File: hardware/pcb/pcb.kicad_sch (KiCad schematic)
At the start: 4 parts, among them U101 BQ7694003DBTR, U102 HCZZ0520-13, U103 HCZZ0520-13, U104 ESP32-C3

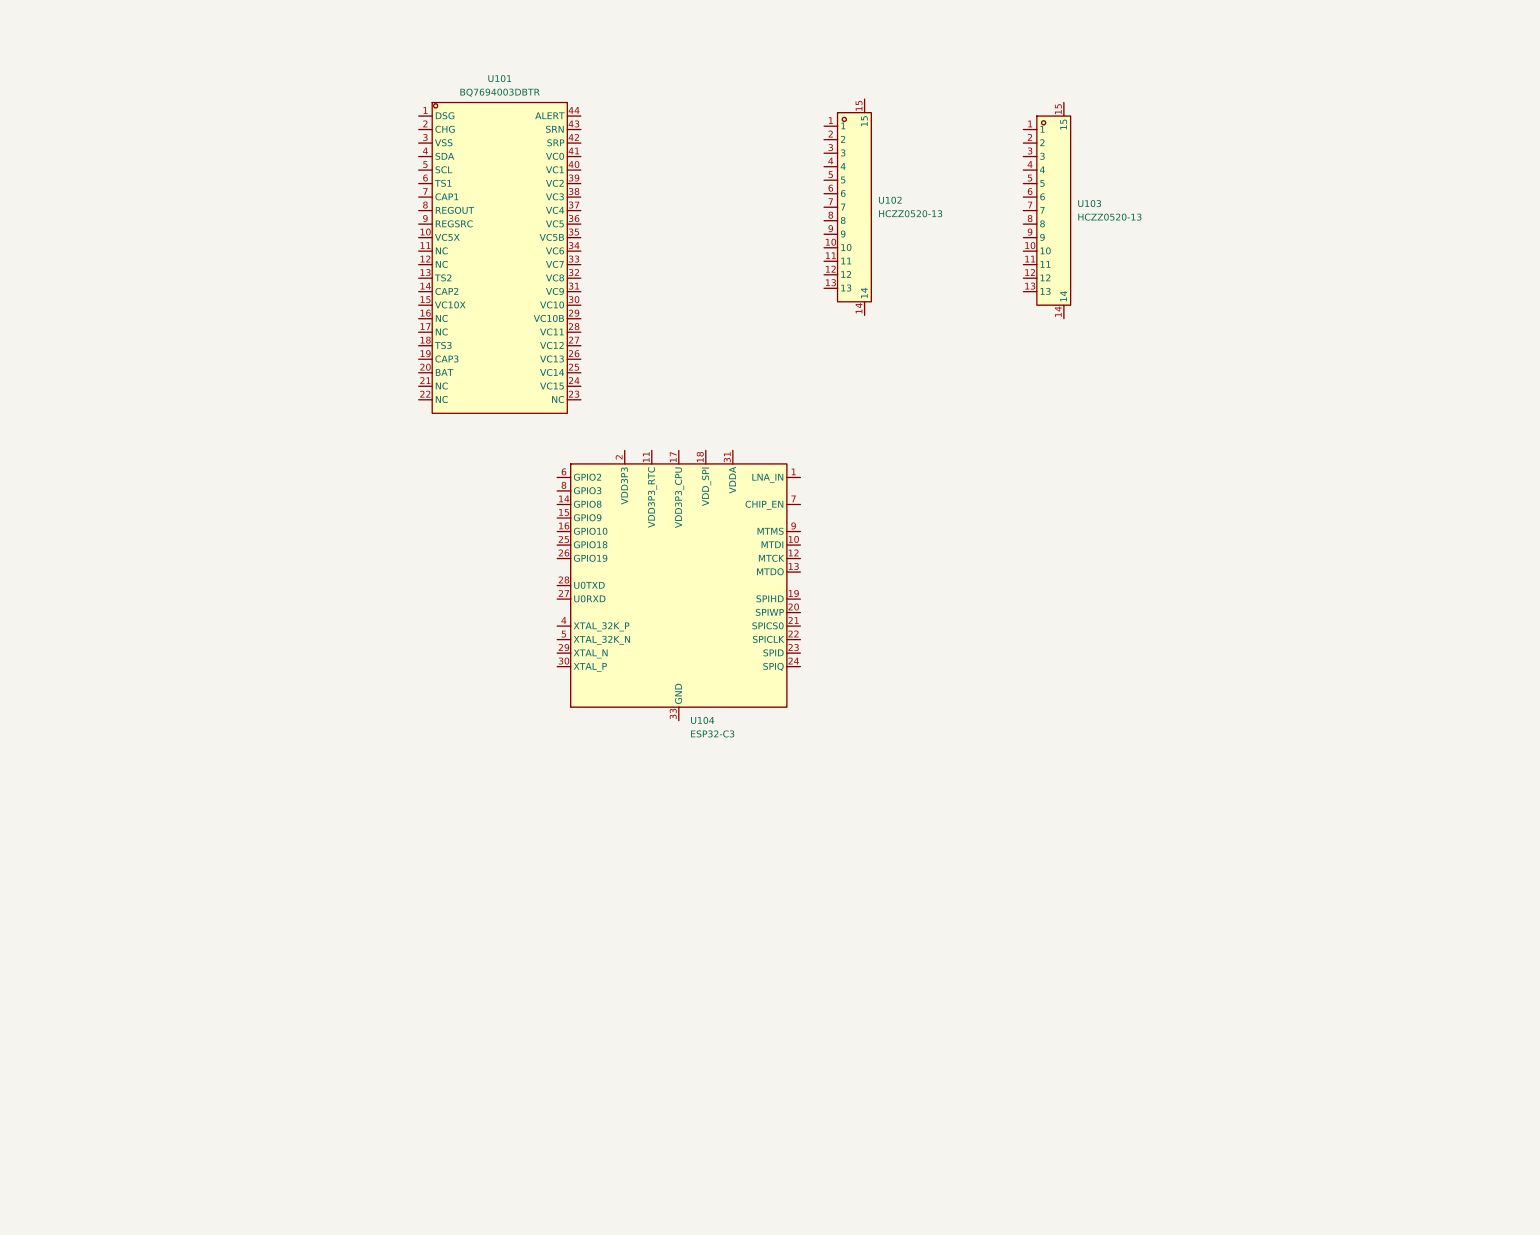
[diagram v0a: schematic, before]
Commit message: re writing the code for better optimization
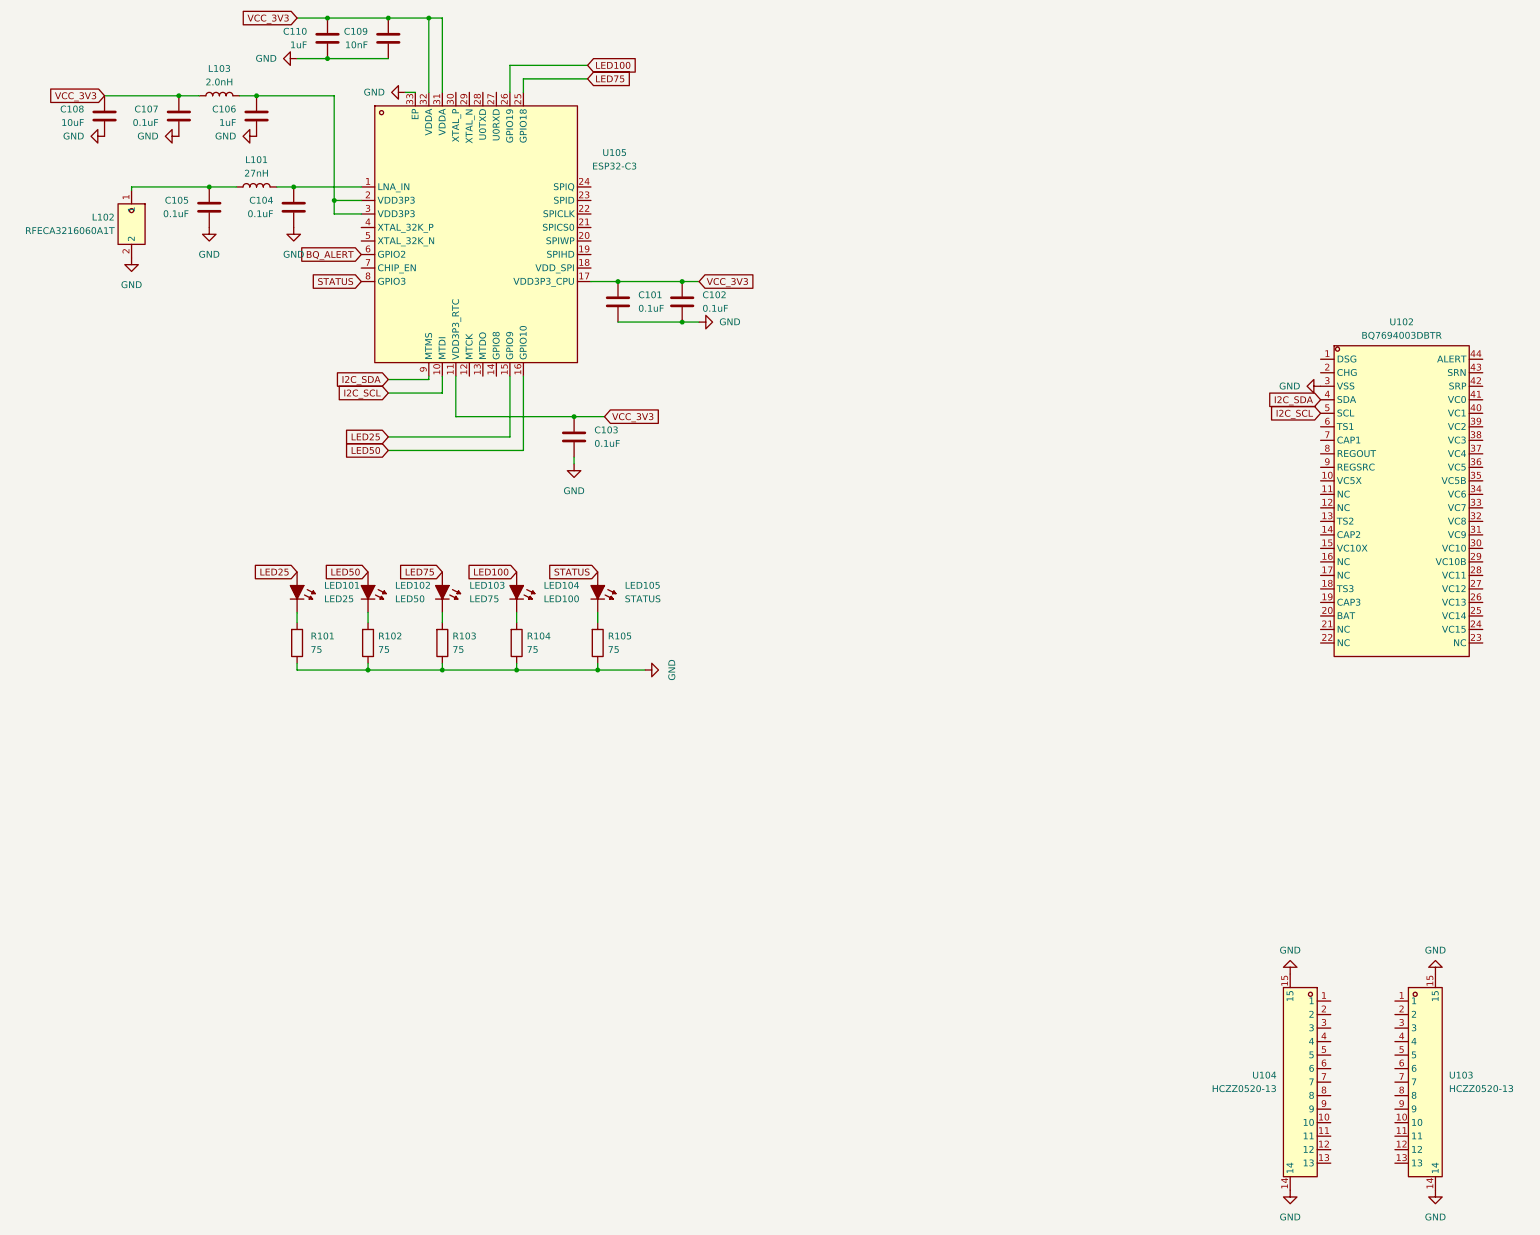
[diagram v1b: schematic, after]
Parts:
- removed U101: BQ7694003DBTR, easyeda2kicad:TSSOP-44_L10.0-W4.4-P0.50-LS6.4-BL-EP, symbol easyeda2kicad:BQ7694003DBTR
- removed U102: HCZZ0520-13, easyeda2kicad:CONN-SMD_13P-P2.50_HCZZ0520-13, symbol easyeda2kicad:HCZZ0520-13
- removed U104: ESP32-C3, Package_DFN_QFN:QFN-32-1EP_5x5mm_P0.5mm_EP3.7x3.7mm, symbol MCU_Espressif:ESP32-C3
- added C101, C102, C103, C104, C105, C107: 0.1uF, PCM_Capacitor_SMD_AKL:C_0402_1005Metric, symbol PCM_Capacitor_AKL:C_0402
- added C106, C110: 1uF, PCM_Capacitor_SMD_AKL:C_0402_1005Metric, symbol PCM_Capacitor_AKL:C_0402
- added C108: 10uF, PCM_Capacitor_SMD_AKL:C_0402_1005Metric, symbol PCM_Capacitor_AKL:C_0402
- added C109: 10nF, PCM_Capacitor_SMD_AKL:C_0402_1005Metric, symbol PCM_Capacitor_AKL:C_0402
- added L101: 27nH, Inductor_SMD:L_1206_3216Metric_Pad1.22x1.90mm_HandSolder, symbol Device:L
- added L102: RFECA3216060A1T, easyeda2kicad:ANT-SMD_L3.1-W1.6, symbol easyeda2kicad:RFECA3216060A1T
- added L103: 2.0nH, Inductor_SMD:L_1206_3216Metric_Pad1.22x1.90mm_HandSolder, symbol Device:L
- added LED101: LED25, PCM_LED_SMD_AKL:LED_0603_1608Metric, symbol PCM_LED_AKL:LED_0603
- added LED102: LED50, PCM_LED_SMD_AKL:LED_0603_1608Metric, symbol PCM_LED_AKL:LED_0603
- added LED103: LED75, PCM_LED_SMD_AKL:LED_0603_1608Metric, symbol PCM_LED_AKL:LED_0603
- added LED104: LED100, PCM_LED_SMD_AKL:LED_0603_1608Metric, symbol PCM_LED_AKL:LED_0603
- added LED105: STATUS, PCM_LED_SMD_AKL:LED_0603_1608Metric, symbol PCM_LED_AKL:LED_0603
- added R101, R102, R103, R104, R105: 75, PCM_Resistor_SMD_AKL:R_0402_1005Metric, symbol PCM_Resistor_AKL:R_0402
- added U102: BQ7694003DBTR, easyeda2kicad:TSSOP-44_L10.0-W4.4-P0.50-LS6.4-BL-EP, symbol easyeda2kicad:BQ7694003DBTR
- added U104: HCZZ0520-13, easyeda2kicad:CONN-SMD_13P-P2.50_HCZZ0520-13, symbol easyeda2kicad:HCZZ0520-13
- added U105: ESP32-C3, easyeda2kicad:QFN-32_L5.0-W5.0-P0.50-TL-EP3.7, symbol easyeda2kicad:ESP32-C3
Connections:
- net GND: now reaches U103.14
- net GND: now also U103.15, C101.2, C102.2, C103.2, C104.2, C105.2, C106.2, C107.2, C108.2, C109.2, C110.2, L102.2, R101.2, R102.2, R103.2, R104.2, R105.2, U102.3 (VSS), U104.14, U104.15, U105.33 (EP)
- new net: LED105.1 (K), R105.1
- new net: LED103.1 (K), R103.1
- new net: C106.1, L103.1, U105.2 (VDD3P3), U105.3 (VDD3P3)
- new net: LED102.1 (K), R102.1
- new net: C104.1, L101.2, U105.1 (LNA_IN)
- new net: C105.1, L101.1, L102.1
- new net: LED101.1 (K), R101.1
- new net: LED104.1 (K), R104.1
- new net BQ_ALERT: U105.6 (GPIO2)
- new net I2C_SCL: U102.5 (SCL), U105.10 (MTDI)
- new net I2C_SDA: U102.4 (SDA), U105.9 (MTMS)
- new net LED100: LED104.2 (A), U105.26 (GPIO19)
- new net LED25: LED101.2 (A), U105.15 (GPIO9)
- new net LED50: LED102.2 (A), U105.16 (GPIO10)
- new net LED75: LED103.2 (A), U105.25 (GPIO18)
- new net STATUS: LED105.2 (A), U105.8 (GPIO3)
- new net VCC_3V3: C101.1, C102.1, C103.1, C107.1, C108.1, C109.1, C110.1, L103.2, U105.11 (VDD3P3_RTC), U105.17 (VDD3P3_CPU), U105.31 (VDDA), U105.32 (VDDA)

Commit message: readme done and eveyrthing done
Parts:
- removed C101, C102, C103, C104, C105, C107: 0.1uF, PCM_Capacitor_SMD_AKL:C_0402_1005Metric, symbol PCM_Capacitor_AKL:C_0402
- removed C106, C110: 1uF, PCM_Capacitor_SMD_AKL:C_0402_1005Metric, symbol PCM_Capacitor_AKL:C_0402
- removed C108: 10uF, PCM_Capacitor_SMD_AKL:C_0402_1005Metric, symbol PCM_Capacitor_AKL:C_0402
- removed C109: 10nF, PCM_Capacitor_SMD_AKL:C_0402_1005Metric, symbol PCM_Capacitor_AKL:C_0402
- removed L101: 27nH, Inductor_SMD:L_1206_3216Metric_Pad1.22x1.90mm_HandSolder, symbol Device:L
- removed L102: RFECA3216060A1T, easyeda2kicad:ANT-SMD_L3.1-W1.6, symbol easyeda2kicad:RFECA3216060A1T
- removed L103: 2.0nH, Inductor_SMD:L_1206_3216Metric_Pad1.22x1.90mm_HandSolder, symbol Device:L
- removed U102: BQ7694003DBTR, easyeda2kicad:TSSOP-44_L10.0-W4.4-P0.50-LS6.4-BL-EP, symbol easyeda2kicad:BQ7694003DBTR
- removed U105: ESP32-C3, easyeda2kicad:QFN-32_L5.0-W5.0-P0.50-TL-EP3.7, symbol easyeda2kicad:ESP32-C3
- added C111, C112, C113: 1uF, Capacitor_SMD:C_0402_1005Metric, symbol PCM_Capacitor_AKL:C_0603
- added C114: 47nF, Capacitor_SMD:C_0402_1005Metric, symbol PCM_Capacitor_AKL:C_0603
- added C118, C119: 1uF, PCM_Capacitor_SMD_AKL:C_0805_2012Metric, symbol PCM_Capacitor_AKL:C_0805
- added C120, C122, C123, C124: 0.1uF, PCM_Capacitor_SMD_AKL:C_0402_1005Metric, symbol PCM_Capacitor_AKL:C_0402
- added C121, C126: 1uF, PCM_Capacitor_SMD_AKL:C_0402_1005Metric, symbol PCM_Capacitor_AKL:C_0402
- added C125: 10nF, PCM_Capacitor_SMD_AKL:C_0402_1005Metric, symbol PCM_Capacitor_AKL:C_0402
- added R106: 100R, PCM_Resistor_SMD_AKL:R_0402_1005Metric, symbol PCM_Resistor_US_AKL:R_0402
- added R107, R108: 4.7k, PCM_Resistor_SMD_AKL:R_0402_1005Metric, symbol PCM_Resistor_US_AKL:R_0402
- added R109, R110: 10k, PCM_Resistor_SMD_AKL:R_0402_1005Metric, symbol PCM_Resistor_US_AKL:R_0402
- added RN101, RN102, RN103: 100R, PCM_Resistor_SMD_AKL:R_Array_Convex_4x0402, symbol PCM_Resistor_US_AKL:R_4x0402_Sep_Convex
- added U101: BQ7695202PFBR, easyeda2kicad:TQFP-48_L7.0-W7.0-P0.50-LS9.0-TL, symbol easyeda2kicad:BQ7695202PFBR
- added U102: MIC5219-3.3YM5, easyeda2kicad:SOT-23-5_L3.0-W1.7-P0.95-LS2.8-TL, symbol easyeda2kicad:MIC5219-3.3YM5
- added U106: ZXTR2012P5-13, easyeda2kicad:POWERDI-5_L5.4-W4.0-LS6.5-RD, symbol easyeda2kicad:ZXTR2012P5-13
- added U107: ESP32-C3-WROOM-02U, RF_Module:ESP32-C3-WROOM-02U, symbol RF_Module:ESP32-C3-WROOM-02U
- U103: value HCZZ0520-13 -> INPUT
- U104: value HCZZ0520-13 -> OUTPUT
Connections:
- net BQ_ALERT: now also R110.2, U101.25 (ALERT), U107.16 (IO2)
- net GND: now also C111.1, C112.1, C113.1, C118.1, C119.2, C120.2, C121.2, C122.2, C123.1, C124.1, C125.1, C126.2, U101.17 (VSS), U101.18 (SRP), U101.20 (SRN), U101.21 (TS1), U101.22 (TS2), U101.23 (TS3), U101.28 (HDQ), U101.29 (CFETOFF), U101.30 (DFETOFF), U101.31 (DCHG), U101.32 (DDSG), U101.33 (RST_SHUT), U102.2 (GND), U106.1 (GND), U107.19 (GND), U107.9 (GND)
- net I2C_SCL: now also R107.1, U101.26 (SCL), U107.4 (IO5)
- net I2C_SDA: now also R108.1, U101.27 (SDA), U107.3 (IO4)
- net LED100: now also U107.13 (IO18)
- net LED25: now also U107.5 (IO6)
- net LED50: now also U107.6 (IO7)
- net LED75: now also U107.10 (IO10)
- net STATUS: now also U107.15 (IO3)
- net VCC_3V3: now also C122.1, C123.2, C124.2, C125.2, R107.2, R108.2, R109.1, R110.1, U102.5 (OUT), U107.1 (3V3)
- net at U104.1: now also U103.1, RN101.8 (R1.2)
- net at U104.10: now also U103.10, RN103.7 (R2.2)
- net at U104.11: now also U103.11, RN103.6 (R3.2)
- net at U104.12: now also U103.12, RN103.5 (R4.2)
- net at U104.13: now also U103.13, R106.1
- net at U104.2: now also U103.2, RN101.7 (R2.2)
- net at U104.3: now also U103.3, RN101.6 (R3.2)
- net at U104.4: now also U103.4, RN101.5 (R4.2)
- net at U104.5: now also U103.5, RN102.8 (R1.2)
- net at U104.6: now also U103.6, RN102.7 (R2.2)
- net at U104.7: now also U103.7, RN102.6 (R3.2)
- net at U104.8: now also U103.8, RN102.5 (R4.2)
- net at U104.9: now also U103.9, RN103.8 (R1.2)
- new net: C126.1, R109.2, U107.2 (EN)
- new net: C111.2, U101.24 (REG18)
- new net: C113.2, U101.34 (REG2)
- new net: C112.2, U101.35 (REG1)
- new net 12V: C118.2, C120.1, C121.1, U102.1 (IN), U102.3 (EN), U106.2 (VOUT)
- new net BATT: C114.1, C114.2, C119.1, R106.2, U101.1 (VC15), U101.2 (VC14), U101.3 (VC13), U101.36 (REGIN), U101.4 (VC12), U101.46 (CP1), U101.47 (BAT), U101.48 (VC16), U106.3 (VIN)
- new net RX: U107.11 (IO20/RXD)
- new net TX: U107.12 (IO21/TXD)
- new net VC00: RN101.1 (R1.1), U101.16 (VC0)
- new net VC01: RN101.2 (R2.1), U101.15 (VC1)
- new net VC02: RN101.3 (R3.1), U101.14 (VC2)
- new net VC03: RN101.4 (R4.1), U101.13 (VC3)
- new net VC04: RN102.1 (R1.1), U101.12 (VC4)
- new net VC05: RN102.2 (R2.1), U101.11 (VC5)
- new net VC06: RN102.3 (R3.1), U101.10 (VC6)
- new net VC07: RN102.4 (R4.1), U101.9 (VC7)
- new net VC08: RN103.1 (R1.1), U101.8 (VC8)
- new net VC09: RN103.2 (R2.1), U101.7 (VC9)
- new net VC10: RN103.3 (R3.1), U101.6 (VC10)
- new net VC11: RN103.4 (R4.1), U101.5 (VC11)
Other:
- moved on the sheet: U103, U104
